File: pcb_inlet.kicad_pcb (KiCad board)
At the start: 2 copper layers, 105 x 70 mm, 12 parts

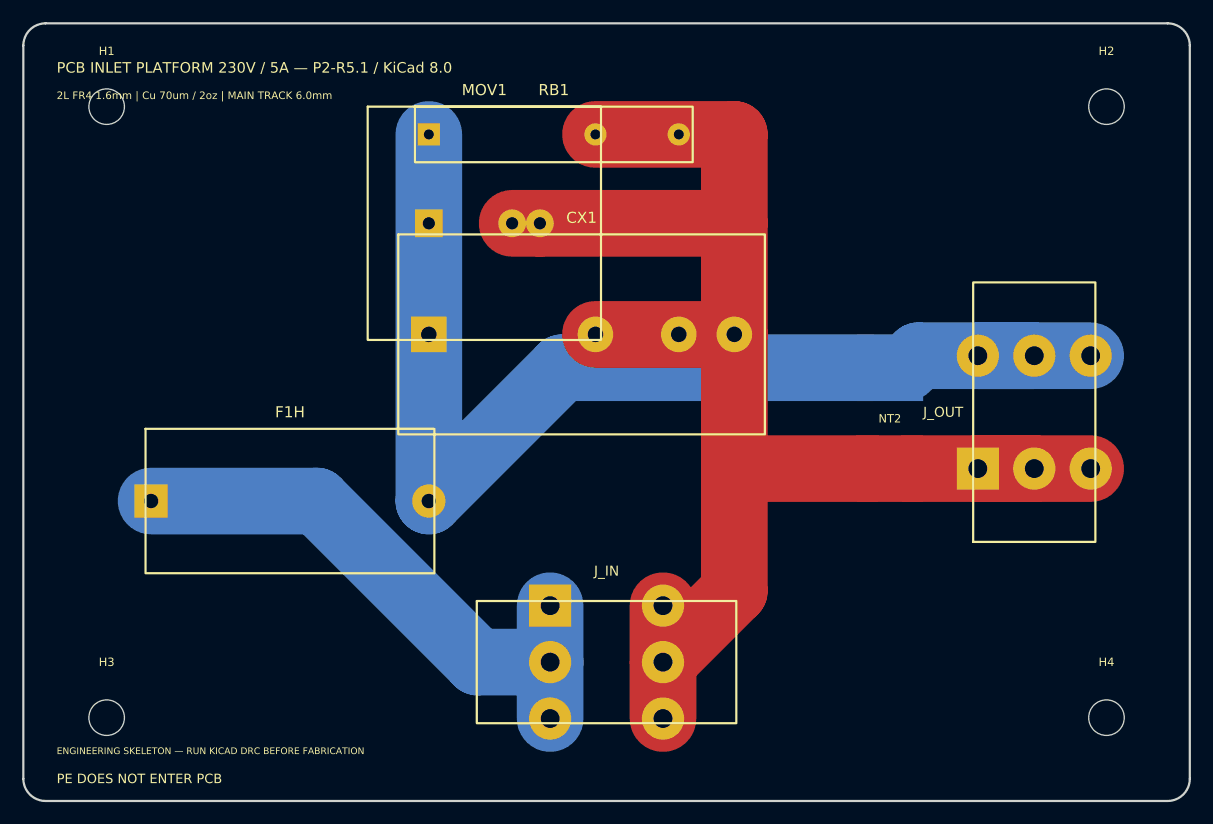
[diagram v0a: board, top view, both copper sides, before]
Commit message: Add files via upload
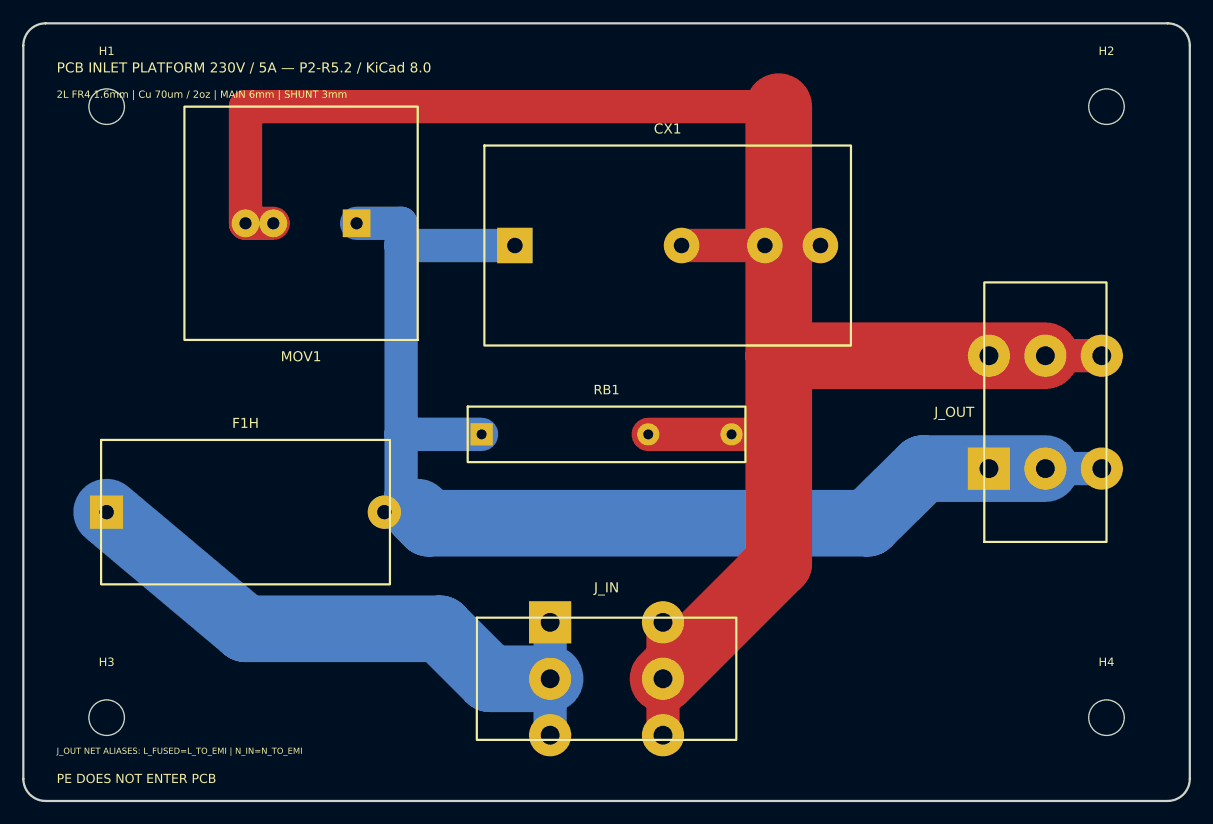
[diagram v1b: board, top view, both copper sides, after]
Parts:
- removed NT1, NT2: NET_TIE, pcb_inlet:NetTie_2_SMD_6mm
- H1, H2, H3, H4: value NPTH 3.2 / 6mm mains hole clearance -> NPTH 3.2 / 6mm mains clearance
- moved RB1 27.4 mm to (52.5, 37.0)
- moved MOV1 16.5 mm to (25.0, 18.0), turned to 180 degrees
- moved CX1 11.1 mm to (58.0, 20.0)
- moved F1H 4.12 mm to (20.0, 44.0)
- moved J_IN 1.50 mm to (52.5, 59.0)
- moved J_OUT 1.00 mm to (92.0, 35.0)
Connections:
- J_OUT pad 1: L_TO_EMI -> L_FUSED
- J_OUT pad 2: N_TO_EMI -> N_IN
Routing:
- net N_IN: track 117.8 -> 185.4 mm
- net L_FUSED: track 78.0 -> 120.2 mm
- net L_TO_EMI: track 22.1 -> 0.00 mm
- net N_TO_EMI: track 21.7 -> 0.00 mm
- net L_IN: track 52.1 -> 55.8 mm
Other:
- board text added: "2L FR4 1.6mm | Cu 70um / 2oz | MAIN 6mm | SHUNT 3mm"
- board text added: "B.Cu LINE | F.Cu NEUTRAL | NO VIAS | NO ZONES"
- board text added: "J_IN WIRE / SERVICE ZONE | MATED DEPTH NORMAL TO PCB >=50mm"
- board text added: "J_OUT NET ALIASES: L_FUSED=L_TO_EMI | N_IN=N_TO_EMI"
- board text added: "J_OUT TO SCHAFNER LINE | MATED DEPTH >=50mm"
- board text added: "PCB INLET PLATFORM 230V / 5A — P2-R5.2 / KiCad 8.0"
- board text removed: "2L FR4 1.6mm | Cu 70um / 2oz | MAIN TRACK 6.0mm"
- board text removed: "B.Cu LINE / F.Cu NEUTRAL / NO VIAS / NO ZONES"
- board text removed: "ENGINEERING SKELETON — RUN KICAD DRC BEFORE FABRICATION"
- board text removed: "J_IN: MATED DEPTH NORMAL TO PCB >=50mm | WIRE EXIT +Y"
- board text removed: "J_OUT: MATED DEPTH NORMAL TO PCB >=50mm | WIRE EXIT TO SCHAFFNER"
- board text removed: "PCB INLET PLATFORM 230V / 5A — P2-R5.1 / KiCad 8.0"
